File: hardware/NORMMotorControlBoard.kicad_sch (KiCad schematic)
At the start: 14 parts, among them J1 Front Left Motor, J2 Front Right Motor, J3 Back Left Motor, J4 Back Right Motor, J5 Conn_01x02_Socket, J6 Conn_01x04_Pin, SW1 Reset, U1 Arduino Nano 33 BLE, U2 Front Motors, U3 Back Motors

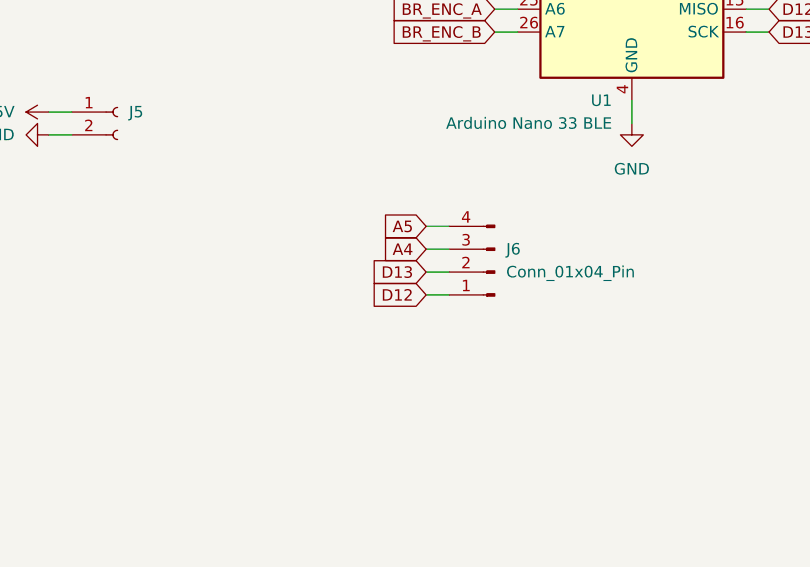
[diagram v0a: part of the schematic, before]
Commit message: Finished V1.0
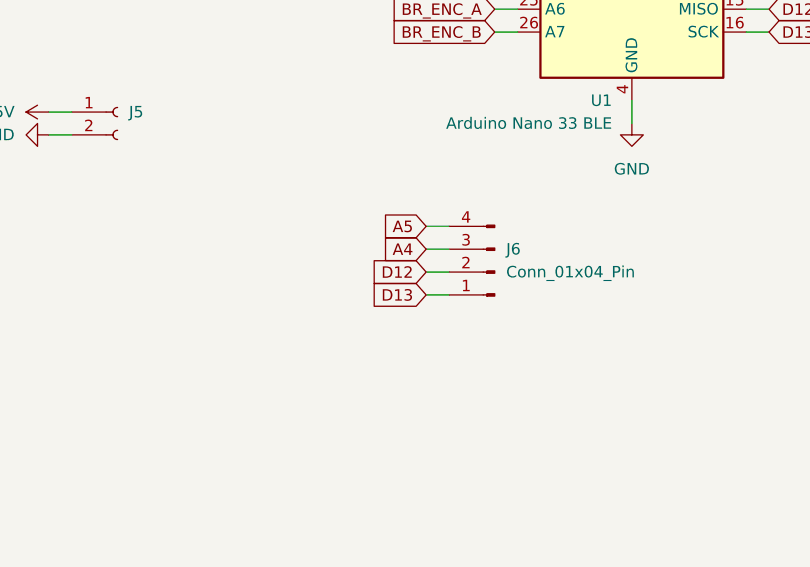
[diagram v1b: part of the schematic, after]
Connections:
- net D12: now also J6.2 (Pin_2); no longer J6.1 (Pin_1)
- net D13: now also J6.1 (Pin_1); no longer J6.2 (Pin_2)
